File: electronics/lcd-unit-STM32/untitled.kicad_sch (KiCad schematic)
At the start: 12 parts, among them J3 Micro_SD_Card

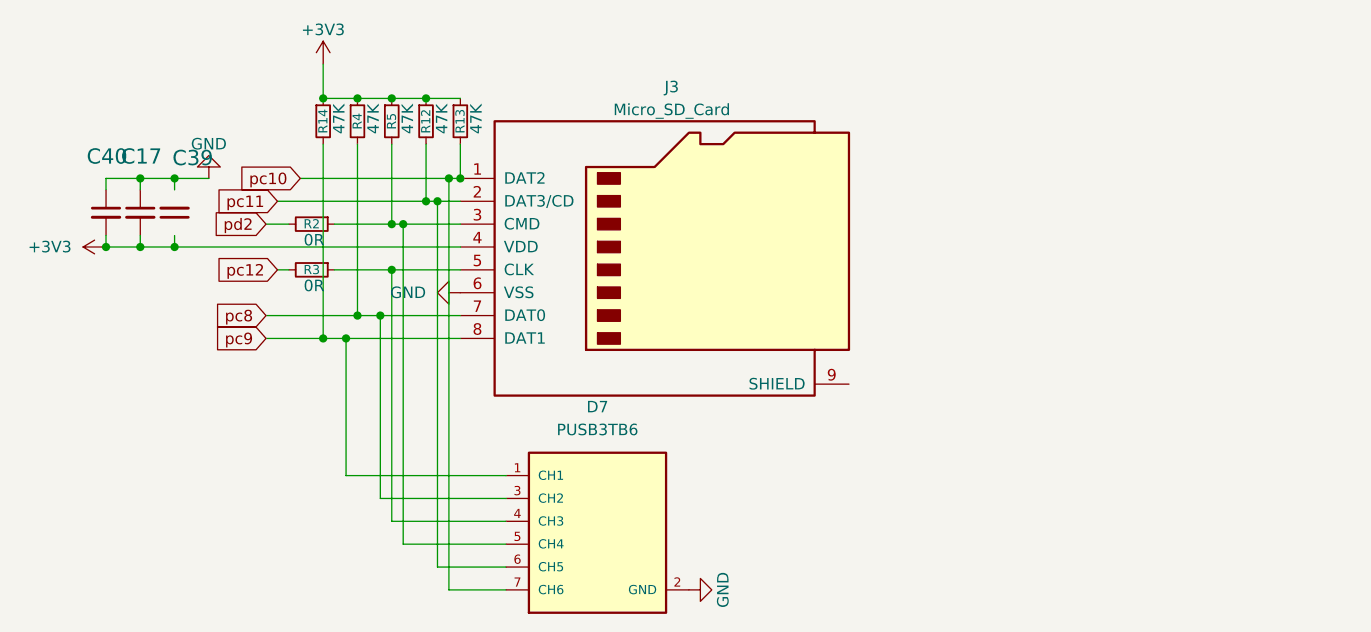
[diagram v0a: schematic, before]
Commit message: uv control fixed
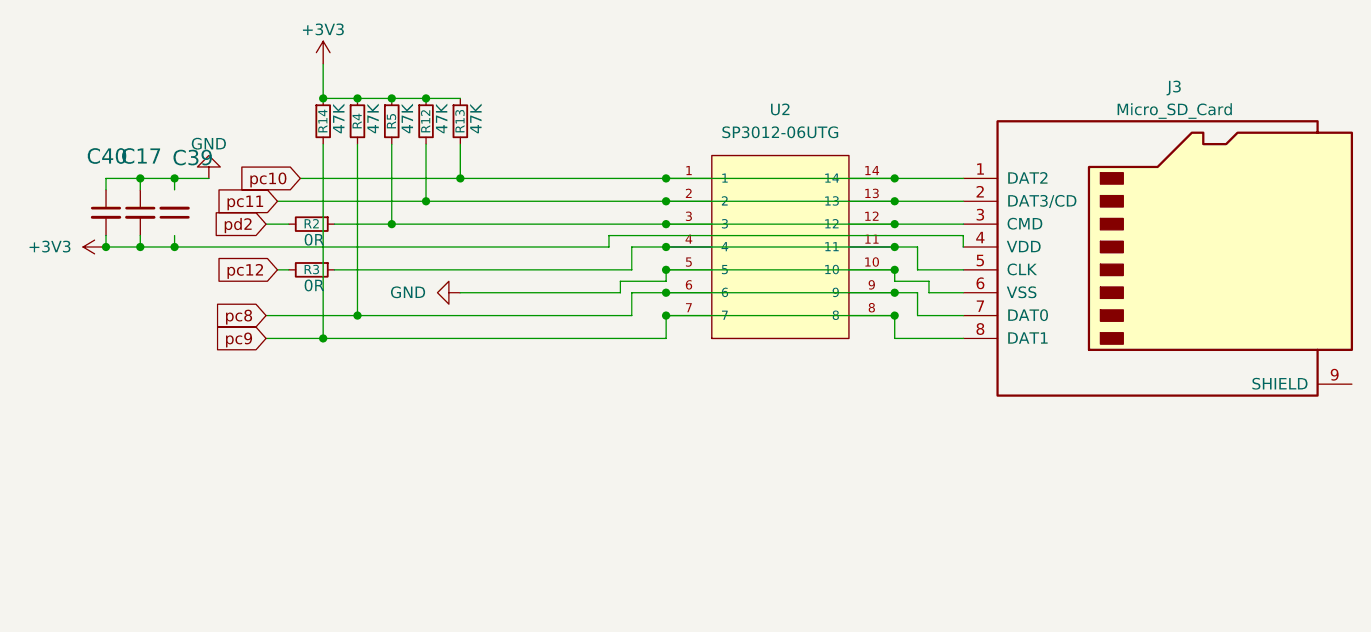
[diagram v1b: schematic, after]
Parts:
- removed D7: PUSB3TB6, moja:pus, symbol moja:PUSB3TB6
- added U2: SP3012-06UTG, moja:SON50P350X135X55-14N, symbol moja:SP3012-06UTG
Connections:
- net GND: now also U2.10, U2.5
- net pc10: now also U2.1, U2.14
- net pc11: now also U2.13, U2.2
- net pc8: now also U2.6, U2.9
- net pc9: now also U2.7, U2.8
- net at J3.3 (CMD), R2.1, R5.2: now also U2.12, U2.3
- net at J3.5 (CLK), R3.1: now also U2.11, U2.4
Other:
- moved on the sheet: J3
